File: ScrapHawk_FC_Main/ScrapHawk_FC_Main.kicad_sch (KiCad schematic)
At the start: 51 parts, among them IC1 MP1584EN-LF-Z, J1 USB_C_Receptacle_USB2.0_16P, J2 Conn_01x06, J3 Conn_01x06, U1 RP2040, U2 W25Q128JVS, U3 AMS1117CD-3.3, U4 LSM6DS3TR, Y1 12M

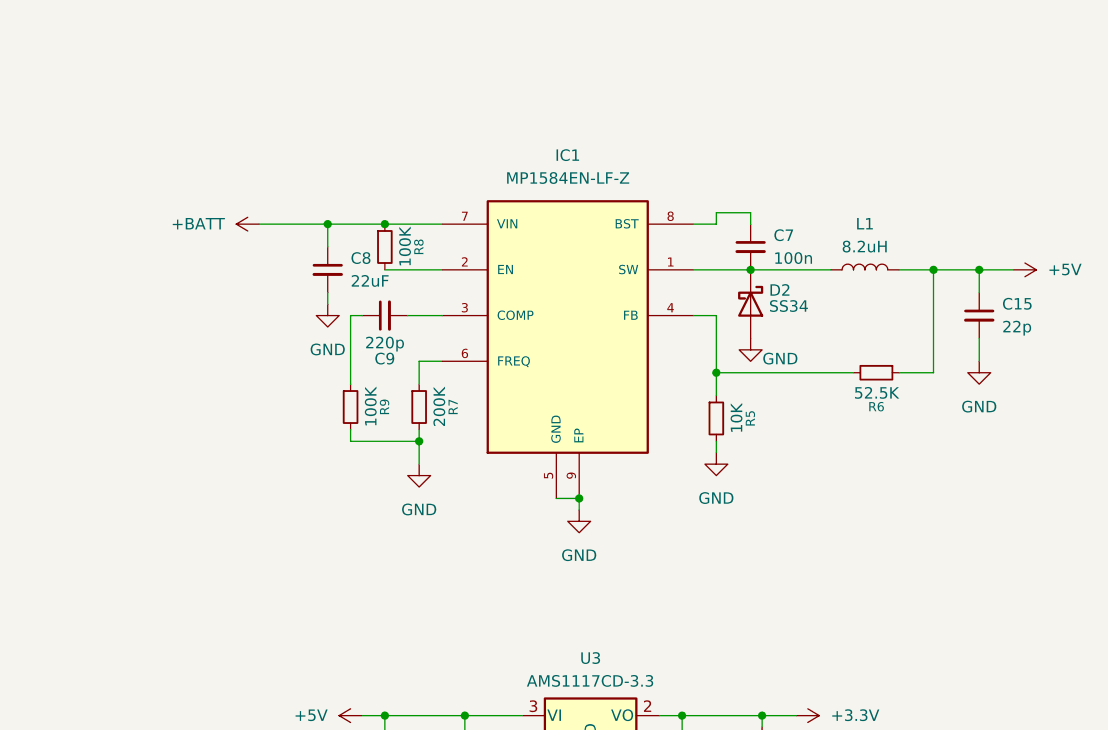
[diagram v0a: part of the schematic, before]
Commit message: update stepdown
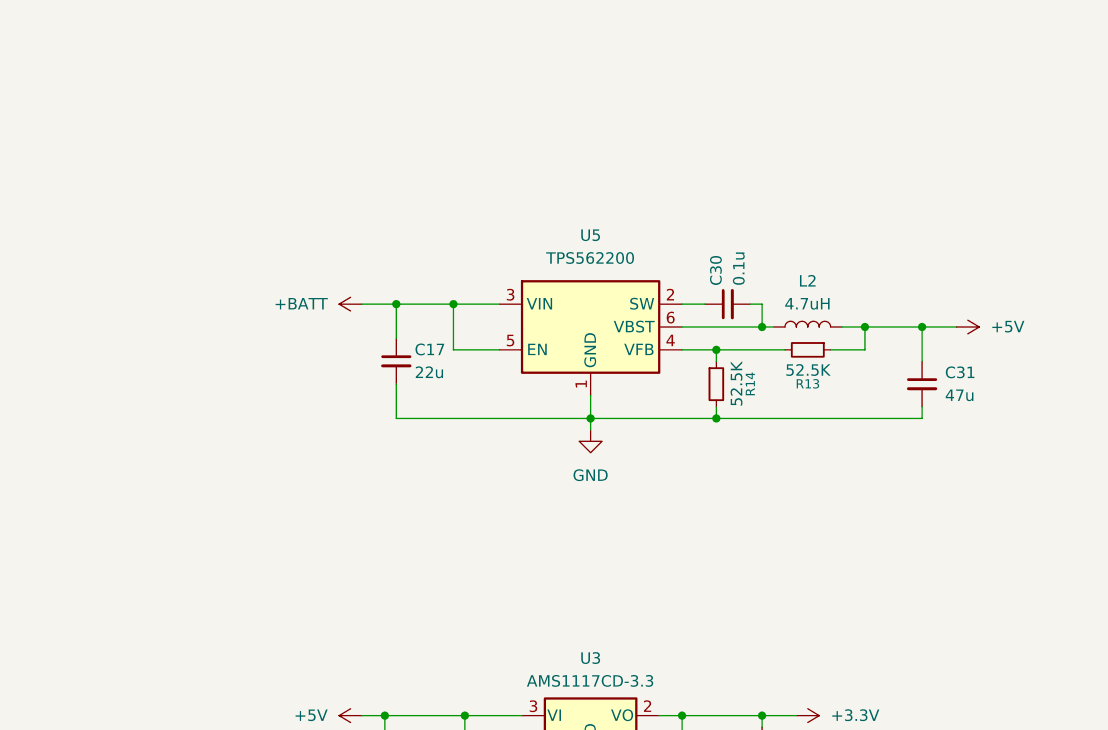
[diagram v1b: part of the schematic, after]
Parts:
- removed C15: 22p, Capacitor_SMD:C_0603_1608Metric, symbol Device:C_Small
- removed C7: 100n, Capacitor_SMD:C_0603_1608Metric, symbol Device:C_Small
- removed C8: 22uF, Capacitor_SMD:C_0603_1608Metric, symbol Device:C_Small
- removed C9: 220p, Capacitor_SMD:C_0603_1608Metric, symbol Device:C_Small
- removed D2: SS34, Diode_SMD:D_SMB_Handsoldering, symbol Device:D_Schottky
- removed IC1: MP1584EN-LF-Z, MP1584EN-LF-Z:SOIC127P600X170-9N, symbol MP1584EN:MP1584EN-LF-Z
- removed L1: 8.2uH, Inductor_SMD:L_Chilisin_BMRA00050520, symbol Device:L
- removed R5: 10K, Resistor_SMD:R_0603_1608Metric, symbol Device:R_Small
- removed R6: 52.5K, Resistor_SMD:R_0603_1608Metric, symbol Device:R_Small
- removed R7: 200K, Resistor_SMD:R_0603_1608Metric, symbol Device:R_Small
- removed R8, R9: 100K, Resistor_SMD:R_0603_1608Metric, symbol Device:R_Small
- added C17: 22u, Capacitor_SMD:C_0603_1608Metric, symbol Device:C_Small
- added C30: 0.1u, Capacitor_SMD:C_0603_1608Metric, symbol Device:C_Small
- added C31: 47u, Capacitor_SMD:C_0603_1608Metric, symbol Device:C_Small
- added L2: 4.7uH, Inductor_SMD:L_Chilisin_BMRA00050520, symbol Device:L
- added R13, R14: 52.5K, Resistor_SMD:R_0603_1608Metric, symbol Device:R_Small
- added U5: TPS562200, Package_TO_SOT_SMD:SOT-23-6, symbol Regulator_Switching:TPS562200
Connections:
- net +5V: now also C31.1, L2.2, R13.1
- net +BATT: now also C17.1, U5.3 (VIN), U5.5 (EN)
- net GND: now also C17.2, C31.2, R14.2, U5.1 (GND)
- new net: R13.2, R14.1, U5.4 (VFB)
- new net: C30.1, U5.2 (SW)
- new net: C30.2, L2.1, U5.6 (VBST)
